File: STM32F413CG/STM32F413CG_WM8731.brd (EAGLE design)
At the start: 54 x 33 mm, 59 parts, among them IC1 STM32F413CGU6, IC2 WM8731SEDS_RV, J2 1503_02, X1 USB-MICROB-SMD

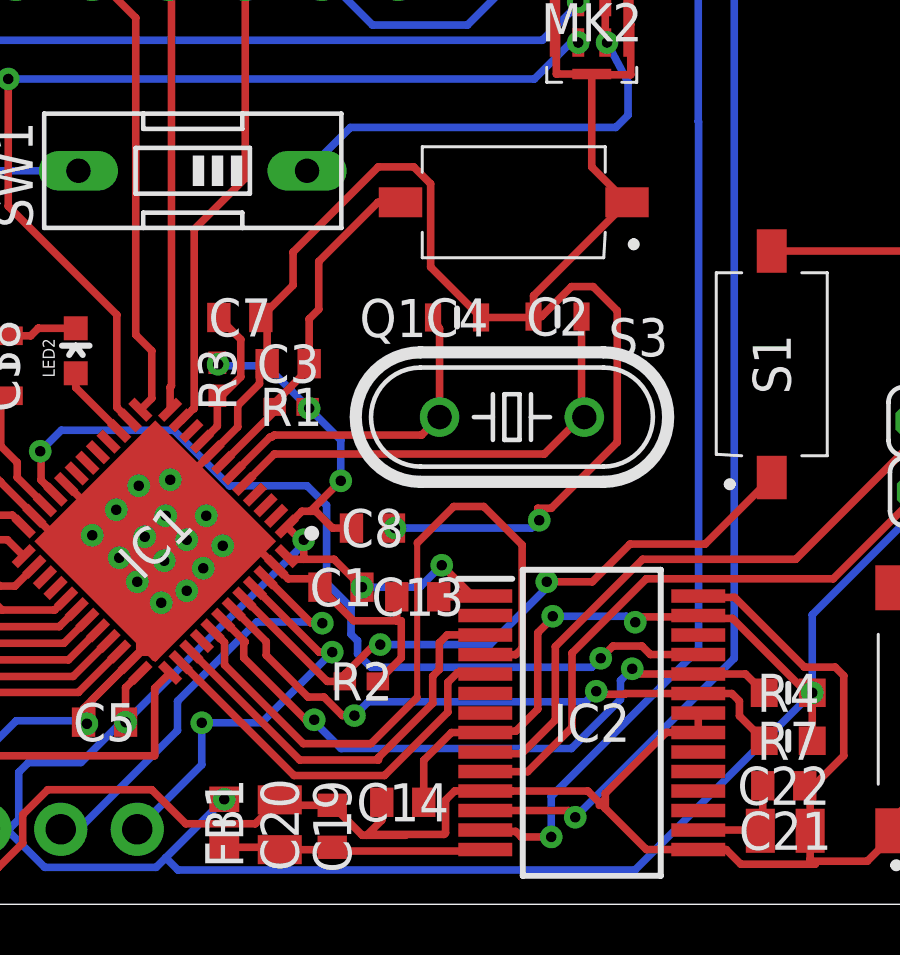
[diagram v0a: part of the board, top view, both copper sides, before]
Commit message: added
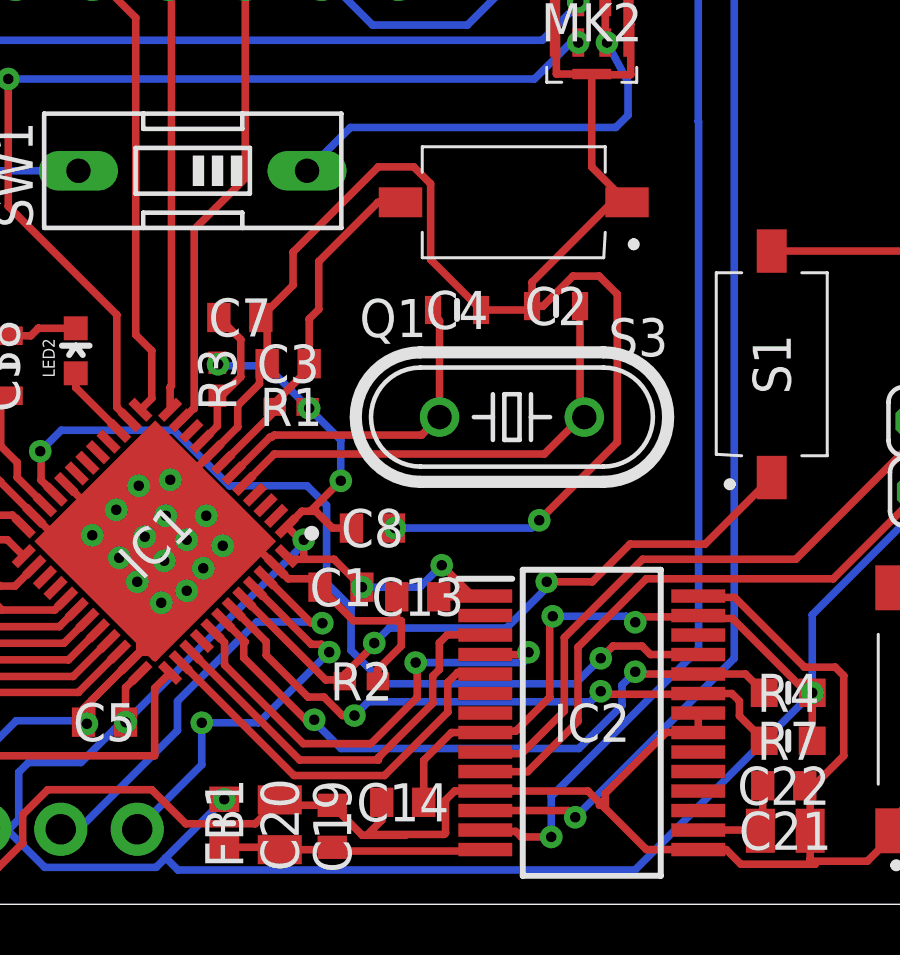
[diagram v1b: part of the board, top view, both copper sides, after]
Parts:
- moved C2 0.35 mm to (31.0, 19.9)
- moved C4 0.25 mm to (27.7, 19.8)
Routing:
- net B5: track 24.4 -> 17.0 mm, vias 0 -> 2
- net B10: track 30.6 -> 31.1 mm
